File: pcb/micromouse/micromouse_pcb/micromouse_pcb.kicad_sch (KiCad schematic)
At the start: 16 parts, among them J1 USB_B_Micro, J2 Conn_01x20_Pin, J3 Conn_01x20_Pin, U2 ESP32-S3-WROOM-1, U3 AMS1117-3.3

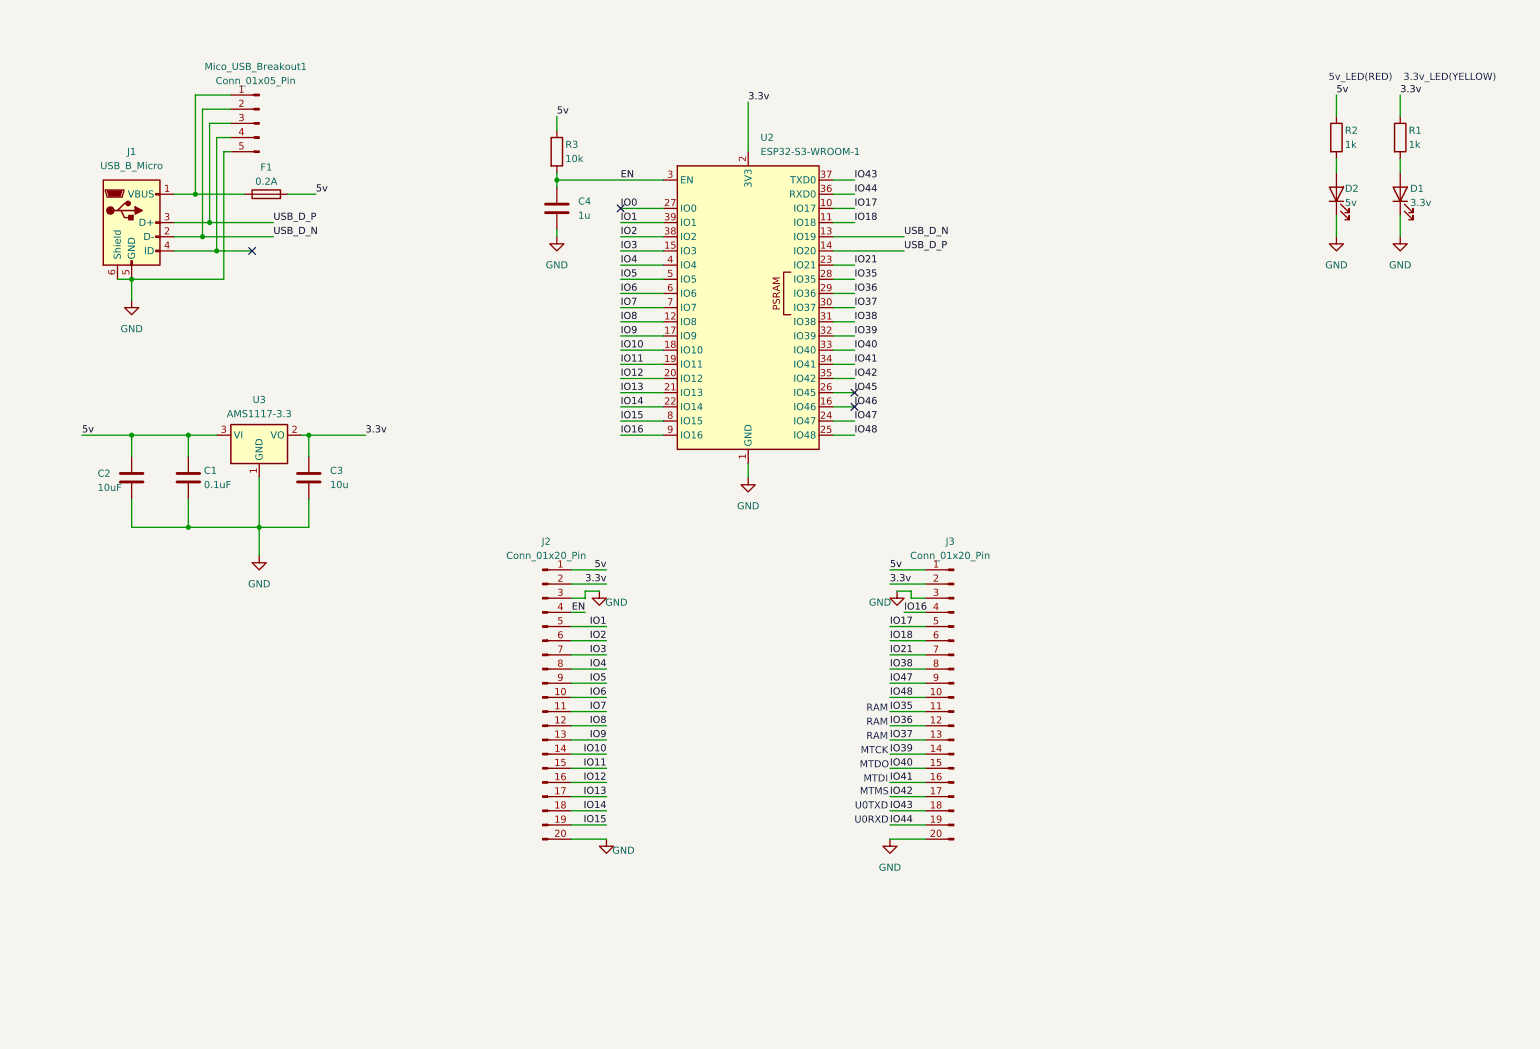
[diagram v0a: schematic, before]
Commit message: pcb progerss clock and breakout_board done
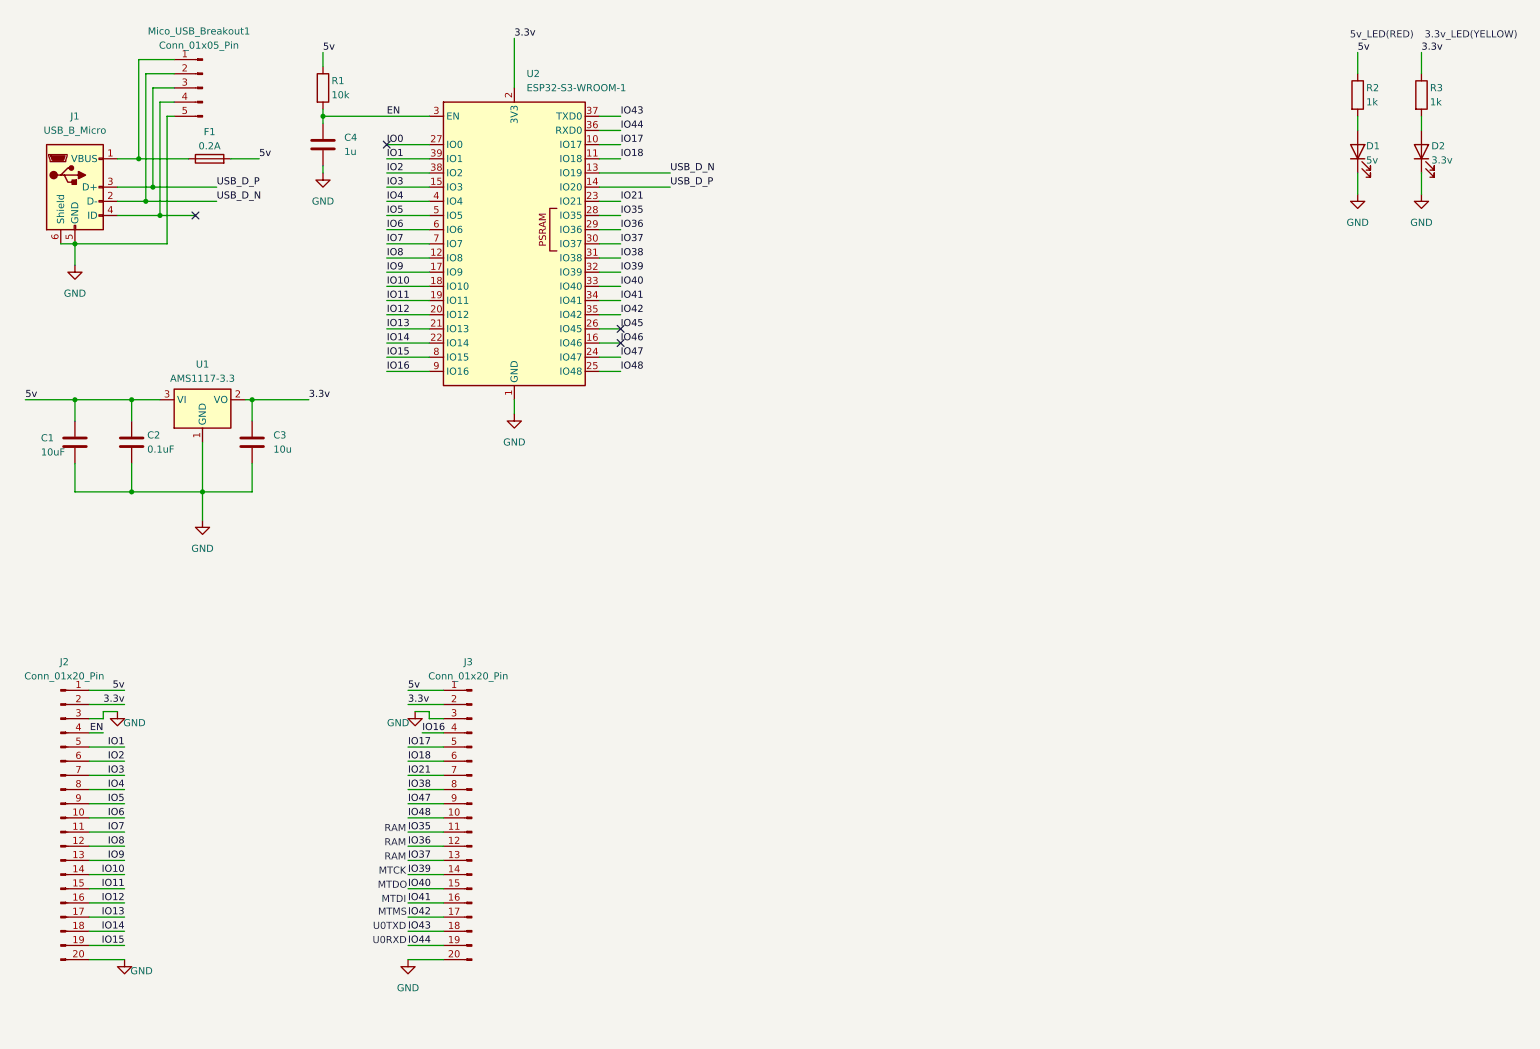
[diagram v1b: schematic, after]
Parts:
- removed U3: AMS1117-3.3, Package_TO_SOT_SMD:SOT-223-3_TabPin2, symbol Regulator_Linear:AMS1117-3.3
- added U1: AMS1117-3.3, Package_TO_SOT_SMD:SOT-223-3_TabPin2, symbol Regulator_Linear:AMS1117-3.3
- C1: value 0.1uF -> 10uF
- C2: value 10uF -> 0.1uF
- D1: value 3.3v -> 5v
- D2: value 5v -> 3.3v
- R1: value 1k -> 10k
- R3: value 10k -> 1k
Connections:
- net 3.3v: now also R3.1, U1.2 (VO); no longer R1.1
- net 5v: now also R1.1, U1.3 (VI); no longer R3.1
- net EN: now also R1.2; no longer R3.2
- net GND: now also U1.1 (GND)
- net at D2.2 (A): now also R3.2; no longer R2.2
- net at D1.2 (A): now also R2.2; no longer R1.2

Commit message: pcb of micromouse done
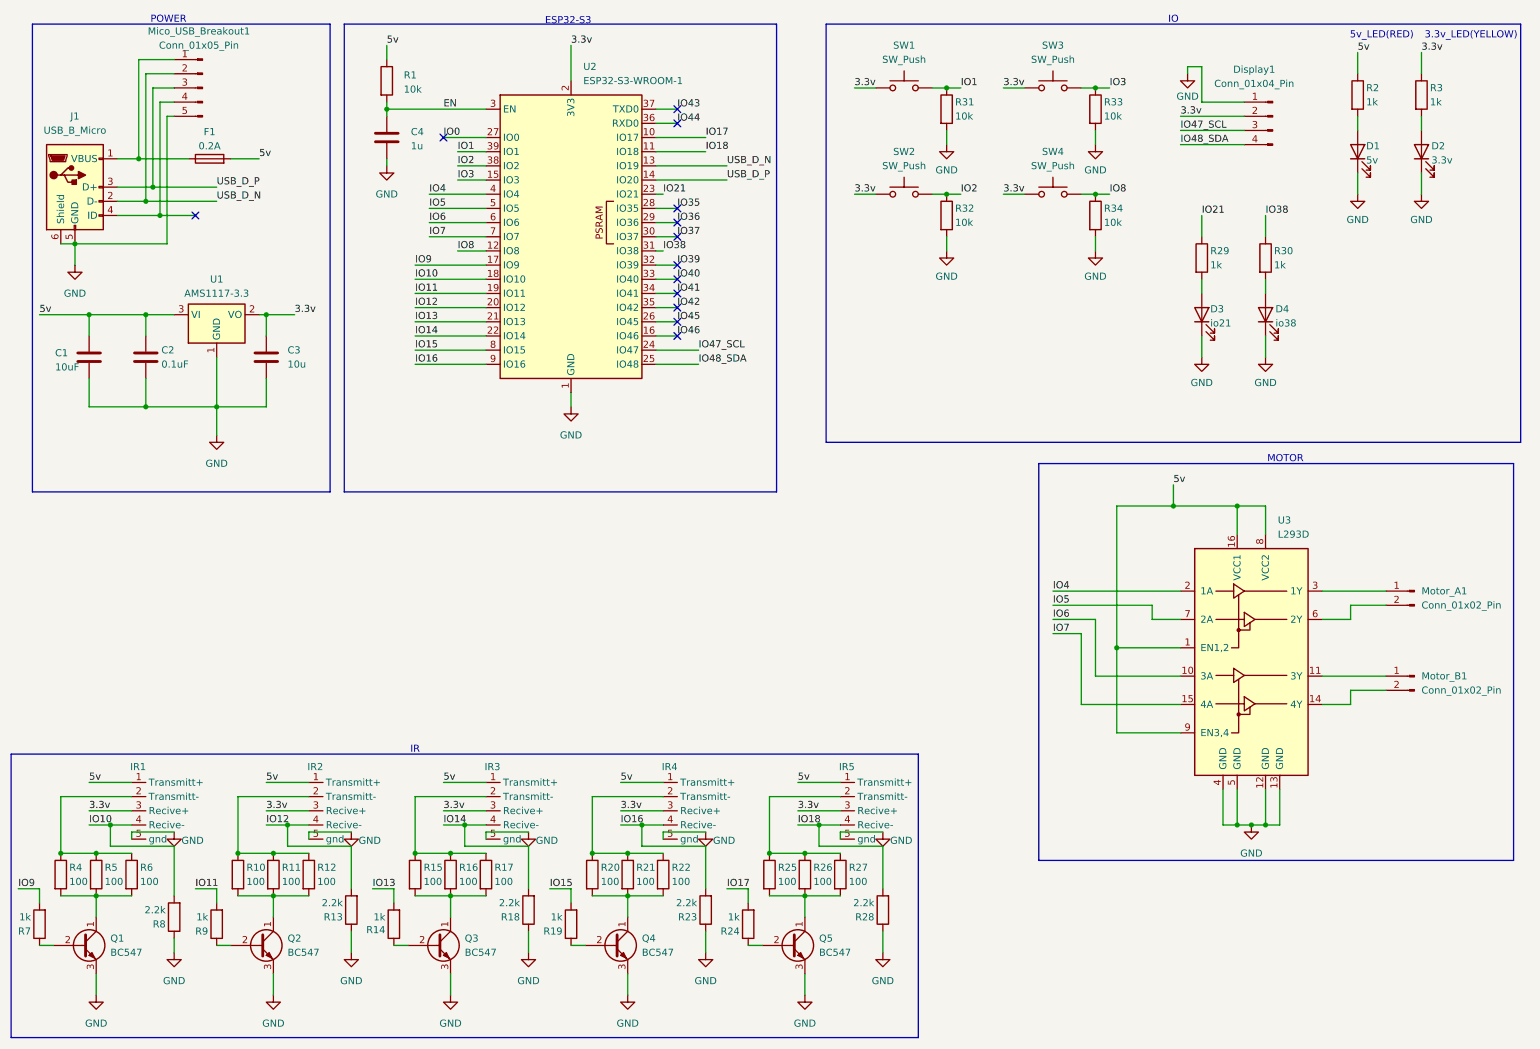
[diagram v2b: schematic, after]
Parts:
- removed J2, J3: Conn_01x20_Pin, Connector_PinHeader_2.54mm:PinHeader_1x20_P2.54mm_Vertical, symbol Connector:Conn_01x20_Pin
- added D3: io21, Ivar_footprint_library:IVAR_0603_SMD_LED, symbol Device:LED
- added D4: io38, Ivar_footprint_library:IVAR_0603_SMD_LED, symbol Device:LED
- added Display1: Conn_01x04_Pin, Ivar_footprint_library:IVAR_OLED_I2C, symbol Connector:Conn_01x04_Pin
- added IR1, IR2, IR3, IR4, IR5: ~, Ivar_footprint_library:IVAR_IR, symbol IVAR_symbol_lbrary:IR_transmitt_recive
- added Motor_A1, Motor_B1: Conn_01x02_Pin, Connector_PinHeader_2.54mm:PinHeader_1x02_P2.54mm_Vertical, symbol Connector:Conn_01x02_Pin
- added Q1, Q2, Q3, Q4, Q5: BC547, Package_TO_SOT_THT:TO-92_Inline, symbol Transistor_BJT:BC547
- added R10, R11, R12, R15, R16, R17, R20, R21, R22, R25, R26, R27, R4, R5, R6: 100, Ivar_footprint_library:IVAR_1206_SMD_R, symbol Device:R
- added R13, R18, R23, R28, R8: 2.2k, Ivar_footprint_library:IVAR_1206_SMD_R, symbol Device:R
- added R14, R19, R24, R29, R30, R7, R9: 1k, Ivar_footprint_library:IVAR_1206_SMD_R, symbol Device:R
- added R31, R32, R33, R34: 10k, Ivar_footprint_library:IVAR_1206_SMD_R, symbol Device:R
- added SW1, SW2, SW3, SW4: SW_Push, Ivar_footprint_library:IVAR_BUTTON_RED_SMD, symbol Switch:SW_Push
- added U3: L293D, Package_DIP:DIP-16_W7.62mm, symbol Driver_Motor:L293D
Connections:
- net 3.3v: now also Display1.2 (Pin_2), IR1.3 (Recive+), IR2.3 (Recive+), IR3.3 (Recive+), IR4.3 (Recive+), IR5.3 (Recive+), SW1.1, SW2.1, SW3.1, SW4.1
- net 5v: now also IR1.1 (Transmitt+), IR2.1 (Transmitt+), IR3.1 (Transmitt+), IR4.1 (Transmitt+), IR5.1 (Transmitt+), U3.1 (EN1,2), U3.16 (VCC1), U3.8 (VCC2), U3.9 (EN3,4)
- net GND: now also D3.1 (K), D4.1 (K), Display1.1 (Pin_1), IR1.5 (gnd), IR2.5 (gnd), IR3.5 (gnd), IR4.5 (gnd), IR5.5 (gnd), Q1.3 (E), Q2.3 (E), Q3.3 (E), Q4.3 (E), Q5.3 (E), R13.1, R18.1, R23.1, R28.1, R31.2, R32.2, R33.2, R34.2, R8.1, U3.12 (GND), U3.13 (GND), U3.4 (GND), U3.5 (GND)
- net IO1: now also R31.1, SW1.2
- net IO10: now also IR1.4 (Recive-), R8.2
- net IO11: now also R9.2
- net IO12: now also IR2.4 (Recive-), R13.2
- net IO13: now also R14.2
- net IO14: now also IR3.4 (Recive-), R18.2
- net IO15: now also R19.2
- net IO16: now also IR4.4 (Recive-), R23.2
- net IO17: now also R24.2
- net IO18: now also IR5.4 (Recive-), R28.2
- net IO2: now also R32.1, SW2.2
- net IO21: now also R29.1
- net IO3: now also R33.1, SW3.2
- net IO38: now also R30.1
- net IO4: now also U3.2 (1A)
- net IO5: now also U3.7 (2A)
- net IO6: now also U3.10 (3A)
- net IO7: now also U3.15 (4A)
- net IO8: now also R34.1, SW4.2
- net IO9: now also R7.2
- net IO47 renamed IO47_SCL
- net IO47_SCL: now also Display1.3 (Pin_3)
- net IO48 renamed IO48_SDA
- net IO48_SDA: now also Display1.4 (Pin_4)
- new net: IR1.2 (Transmitt-), R4.1, R5.1, R6.1
- new net: Q5.2 (B), R24.1
- new net: IR3.2 (Transmitt-), R15.1, R16.1, R17.1
- new net: Motor_B1.1 (Pin_1), U3.11 (3Y)
- new net: Motor_B1.2 (Pin_2), U3.14 (4Y)
- new net: Q3.2 (B), R14.1
- new net: D3.2 (A), R29.2
- new net: IR5.2 (Transmitt-), R25.1, R26.1, R27.1
- new net: Q5.1 (C), R25.2, R26.2, R27.2
- new net: IR4.2 (Transmitt-), R20.1, R21.1, R22.1
- new net: Q4.1 (C), R20.2, R21.2, R22.2
- new net: Q3.1 (C), R15.2, R16.2, R17.2
- new net: Q1.1 (C), R4.2, R5.2, R6.2
- new net: Q1.2 (B), R7.1
- new net: Q4.2 (B), R19.1
- new net: IR2.2 (Transmitt-), R10.1, R11.1, R12.1
- new net: Q2.1 (C), R10.2, R11.2, R12.2
- new net: Q2.2 (B), R9.1
- new net: Motor_A1.1 (Pin_1), U3.3 (1Y)
- new net: Motor_A1.2 (Pin_2), U3.6 (2Y)
- new net: D4.2 (A), R30.2
- no-connect marks 4 -> 13
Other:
- note added: "ESP32-S3"
- note added: "IO"
- note added: "IR"
- note added: "MOTOR"
- note added: "POWER"
- note removed: "MTCK"
- note removed: "MTDI"
- note removed: "MTDO"
- note removed: "MTMS"
- note removed: "RAM"
- note removed: "U0RXD"
- note removed: "U0TXD"
- moved on the sheet: C1, C2, C3, C4, R1, U1, U2
